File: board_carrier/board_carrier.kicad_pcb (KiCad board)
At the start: 2 copper layers, 45.1 x 23.5 mm, 13 parts, among them J1 Conn_01x08, J2 Conn_01x08, J3 Conn_01x04, U1 TJA1051T-3, U2 LM78M05_TO252

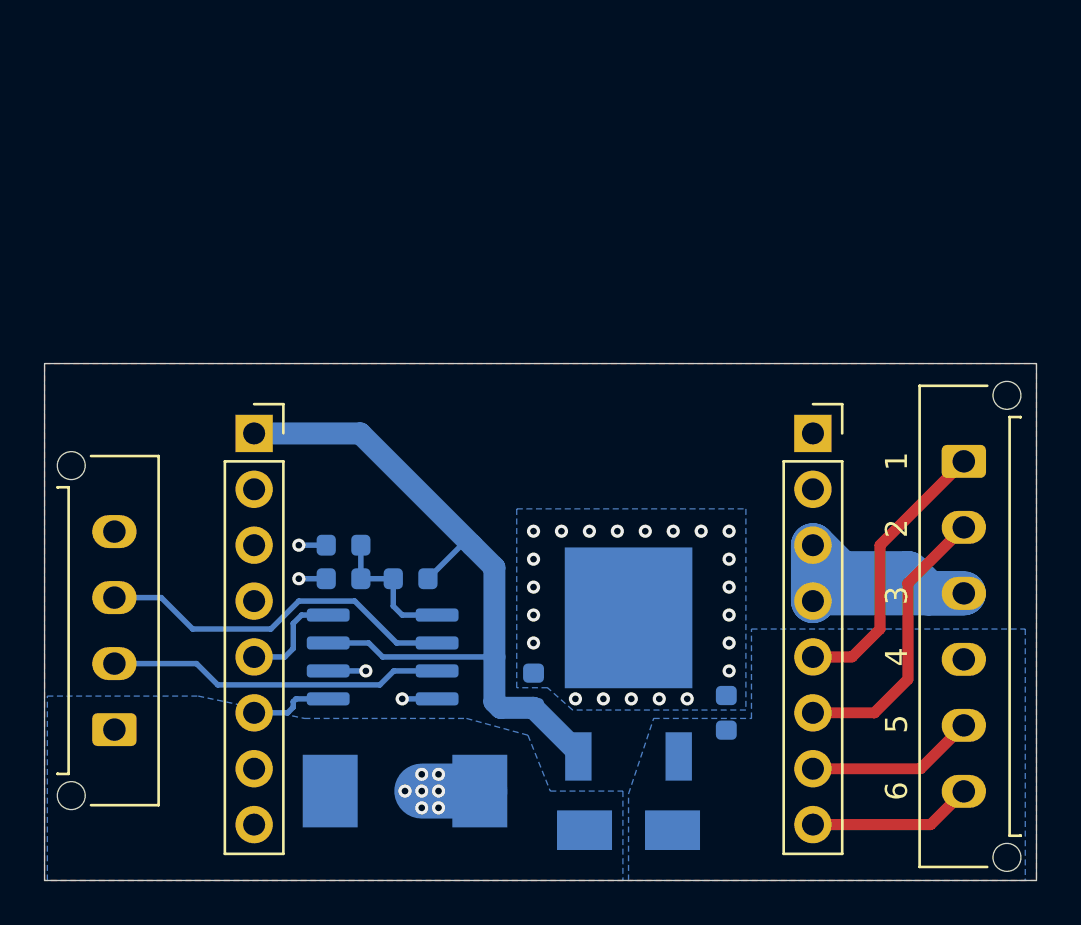
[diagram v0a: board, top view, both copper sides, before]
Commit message: carrier with mx120
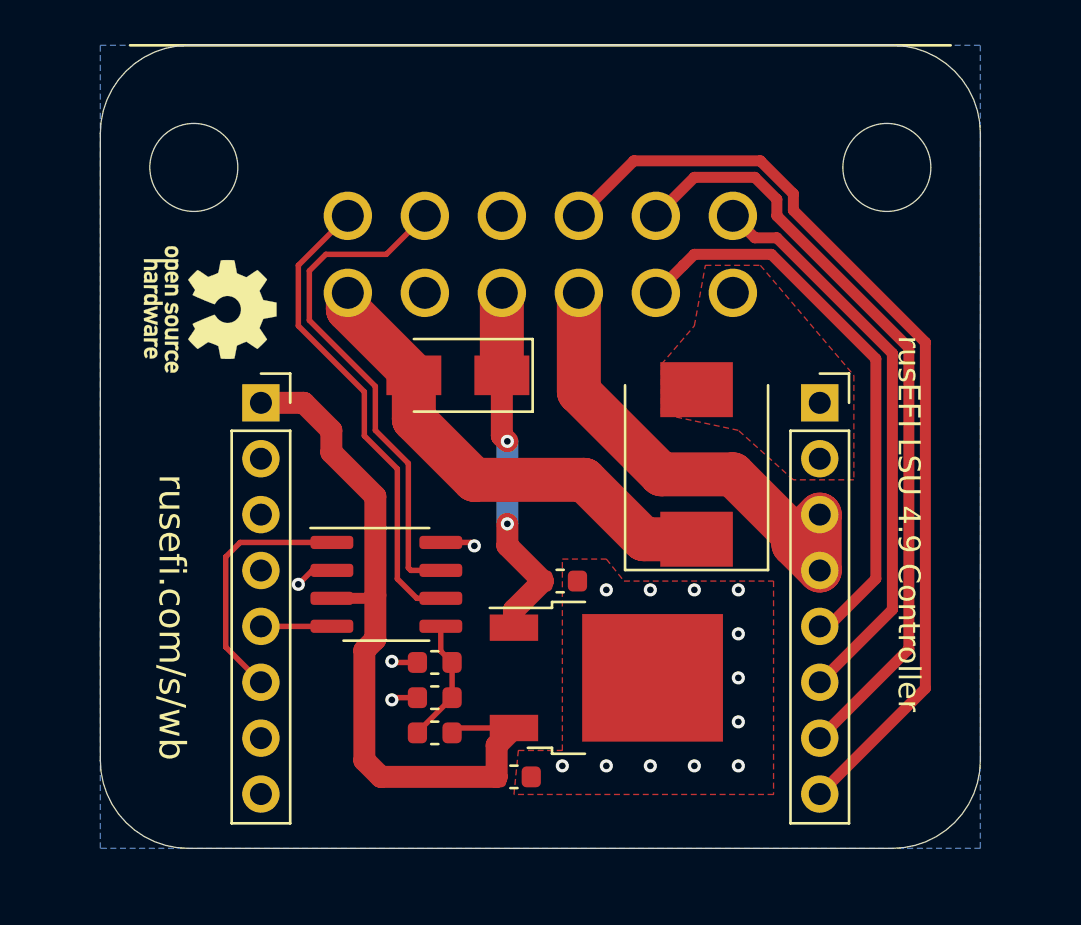
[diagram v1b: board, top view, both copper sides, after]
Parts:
- removed J_LSU1: Conn_01x06, Connector_Molex:Molex_Micro-Fit_3.0_43650-0615_1x06_P3.00mm_Vertical
- added REF**: OSHW-Logo_5.7x6mm_SilkScreen, Symbol:OSHW-Logo_5.7x6mm_SilkScreen, F.Cu at (45.0, 66.8)
- C1, C2, C3, D1, D2, R1, R2, U1, U2: moved to F.Cu
- J3: value Conn_01x04 -> Conn_02x06_Top_Bottom; footprint Connector_Molex:Molex_Micro-Fit_3.0_43650-0415_1x04_P3.00mm_Vertical -> mx120:mx120g-12
- moved J3 27.7 mm to (60.0, 66.0), turned to 0 degrees
- moved D2 22.1 mm to (56.2, 69.8)
- moved D1 19.9 mm to (67.1, 73.8), turned to 90 degrees
- moved C1 9.64 mm to (60.9, 79.1), turned to 0 degrees
- moved C3 8.08 mm to (55.2, 84.4)
- moved R1 7.09 mm to (55.2, 86.0)
- moved R2 5.63 mm to (55.2, 82.8)
- moved C2 4.03 mm to (58.8, 88.0), turned to 0 degrees
- moved U1 3.30 mm to (53.0, 79.2)
- moved J2 1.42 mm to (72.7, 71.0)
- moved J1 1.42 mm to (47.3, 71.0)
- moved U2 1.19 mm to (63.0, 83.5), turned to 0 degrees
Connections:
- J3 pad 1: 12V_RAW -> GND
- J3 pad 2: /CAN_H -> /LSU_Ip
- J3 pad 3: /CAN_L -> /LSU_Heater-
- J3 pad 4: GND -> /LSU_Heater+
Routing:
- net /LSU_Un: track 7.48 -> 43.2 mm
- net /LSU_Rtrim: track 7.67 -> 35.3 mm
- net 12V_RAW: track 0.00 -> 22.1 mm
- net /LSU_Heater+: track 0.00 -> 16.5 mm, vias 0 -> 2
- net /LSU_Ip: track 12.8 -> 26.1 mm
- net /LSU_Vm: track 12.9 -> 26.2 mm
- net /CAN_H: track 15.3 -> 23.2 mm
- net /CAN_TX: track 3.78 -> 11.5 mm
- net /LSU_Heater-: track 17.3 -> 23.2 mm
- net /CAN_L: track 16.6 -> 21.6 mm
- net GND: track 8.43 -> 5.76 mm, vias 33 -> 16
- net /CAN_RX: track 4.83 -> 3.23 mm
- net +5V: track 34.9 -> 33.6 mm
- net Net-(C3-Pad1): track 6.40 -> 5.71 mm
- removed copper zone on B.Cu, net /LSU_Heater+
- removed copper zone on B.Cu, net 12V_RAW
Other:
- board size 45.1 x 23.5 mm -> 40 x 36.5 mm
- board text added: "12V"
- board text added: "CAN"
- board text added: "GND"
- board text added: "H"
- board text added: "L"
- board text added: "LSU 4.9"
- board text added: "rusEFI LSU 4.9 Controller"
- board text added: "rusefi.com/s/wb"
- board text removed: "LSU 4.9 ONLY"
